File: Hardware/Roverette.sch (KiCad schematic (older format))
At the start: 4 parts, among them M1 Motor_DC, M2 Motor_DC

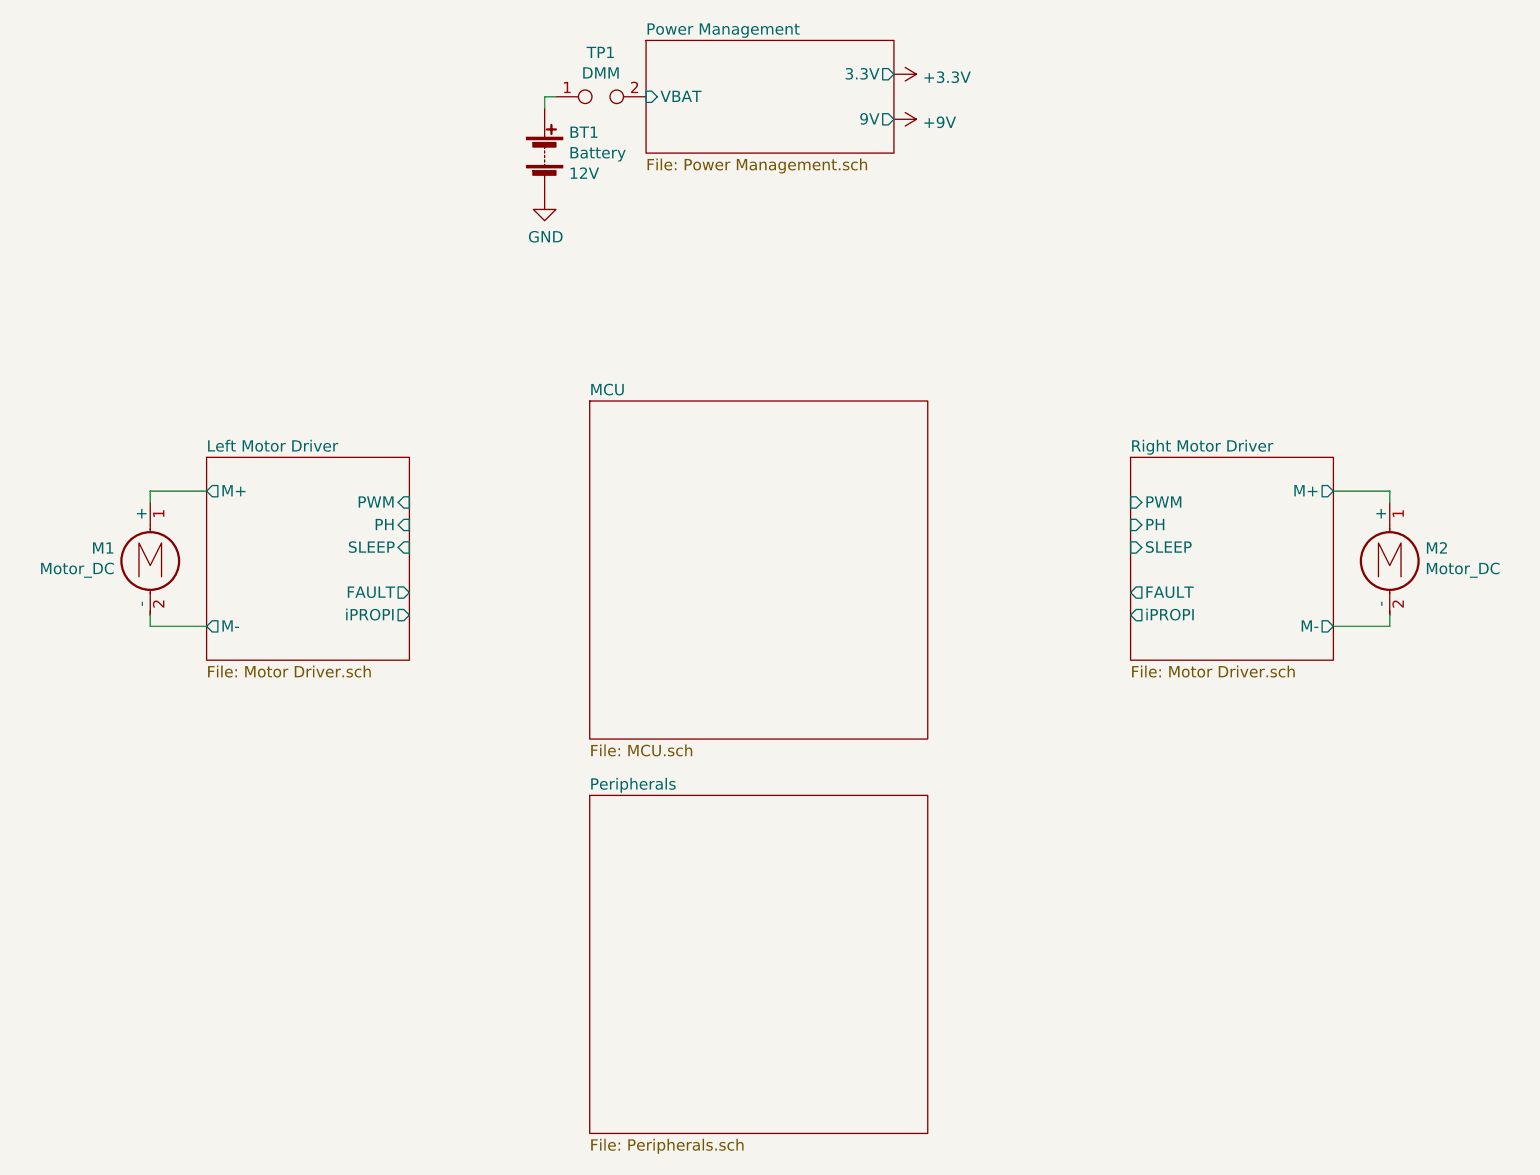
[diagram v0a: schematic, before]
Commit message: Signed-off-by: Usman Mehmood <usmanmehmood55@gmail.com>
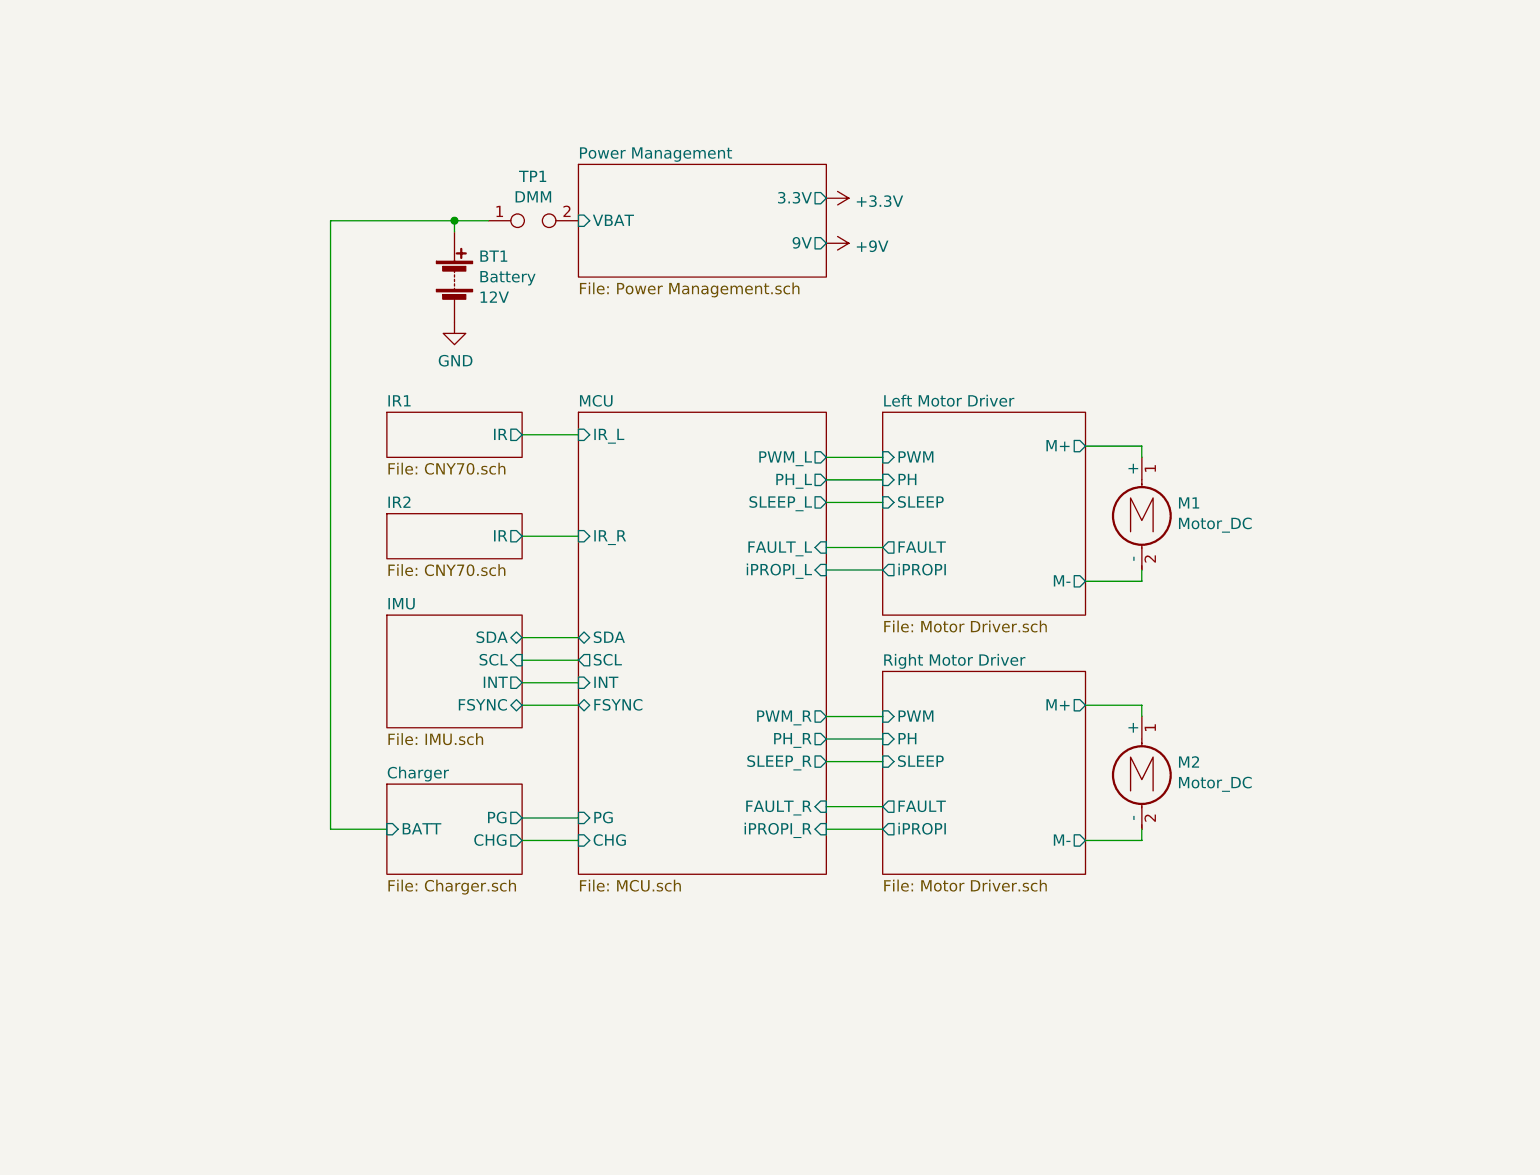
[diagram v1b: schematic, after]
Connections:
- net Charger/BATT: now reaches BT1.1 (+), TP1.1
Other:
- moved on the sheet: BT1, M1, M2, TP1

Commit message: Schematic and readme updated
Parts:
- TP1: symbol Connector:TestPoint_2Pole -> Device:Jumper
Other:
- moved on the sheet: BT1
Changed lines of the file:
@@
 $EndComp
 Wire Wire Line
-	4450 2300 4450 2350
+	4350 2300 4350 2350
 $Comp
-L Connector:TestPoint_2Pole TP1
+L Device:Jumper TP1
 U 1 1 5FF3E3D0
-P 4800 2300
+P 4700 2300
 AR Path="/5FF3E3D0" Ref="TP1"  Part="1"
 AR Path="/5FF0069C/5FF3E3D0" Ref="TP?"  Part="1"
-F 0 "TP1" H 4800 2495 50  0000 C CNN
-F 1 "TestPoint_2Pole" H 4800 2404 50  0001 C CNN
-F 2 "TestPoint:TestPoint_2Pads_Pitch2.54mm_Drill0.8mm" H 4800 2300 50  0001 C CNN
-F 3 "~" H 4800 2300 50  0001 C CNN
-F 4 "DMM" H 4800 2404 50  0000 C CNN "Field4"
-	1    4800 2300
+F 0 "TP1" H 4700 2550 50  0000 C CNN
+F 1 "TestPoint_2Pole" H 4700 2404 50  0001 C CNN
+F 2 "TestPoint:TestPoint_2Pads_Pitch2.54mm_Drill0.8mm" H 4700 2300 50  0001 C CNN
+F 3 "~" H 4700 2300 50  0001 C CNN
+F 4 "DMM" H 4700 2450 50  0000 C CNN "Field4"
+	1    4700 2300
 	1    0    0    -1
 $EndComp
@@
 L power:GND #PWR03
 U 1 1 5FF31DAB
-P 4450 2750
-F 0 "#PWR03" H 4450 2500 50  0001 C CNN
-F 1 "GND" H 4455 2577 50  0000 C CNN
-F 2 "" H 4450 2750 50  0001 C CNN
-F 3 "" H 4450 2750 50  0001 C CNN
-	1    4450 2750
+P 4350 2750
+F 0 "#PWR03" H 4350 2500 50  0001 C CNN
+F 1 "GND" H 4355 2577 50  0000 C CNN
+F 2 "" H 4350 2750 50  0001 C CNN
+F 3 "" H 4350 2750 50  0001 C CNN
+	1    4350 2750
 	1    0    0    -1
 $EndComp
@@
 L Device:Battery BT1
 U 1 1 5FF30336
-P 4450 2550
-F 0 "BT1" H 4558 2641 50  0000 L CNN
-F 1 "Battery" H 4558 2550 50  0000 L CNN
-F 2 "" V 4450 2610 50  0001 C CNN
-F 3 "~" V 4450 2610 50  0001 C CNN
-F 4 "12V" H 4558 2459 50  0000 L CNN "Field4"
-	1    4450 2550
+P 4350 2550
+F 0 "BT1" H 4458 2641 50  0000 L CNN
+F 1 "Battery" H 4458 2550 50  0000 L CNN
+F 2 "" V 4350 2610 50  0001 C CNN
+F 3 "~" V 4350 2610 50  0001 C CNN
+F 4 "12V" H 4458 2459 50  0000 L CNN "Field4"
+	1    4350 2550
 	1    0    0    -1
 $EndComp
@@
 Wire Wire Line
 	6350 3350 6100 3350
-Connection ~ 4450 2300
-Wire Wire Line
-	4450 2300 3900 2300
-Wire Wire Line
-	4450 2300 4600 2300
 $Sheet
 S 5000 2050 1100 500
@@
 F4 "9V" O R 6100 2400 50
 $EndSheet
+Wire Wire Line
+	4350 2300 3900 2300
+Wire Wire Line
+	4400 2300 4350 2300
+Connection ~ 4350 2300
 $EndSCHEMATC
